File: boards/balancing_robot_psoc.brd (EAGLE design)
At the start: 35 x 75 mm, 31 parts

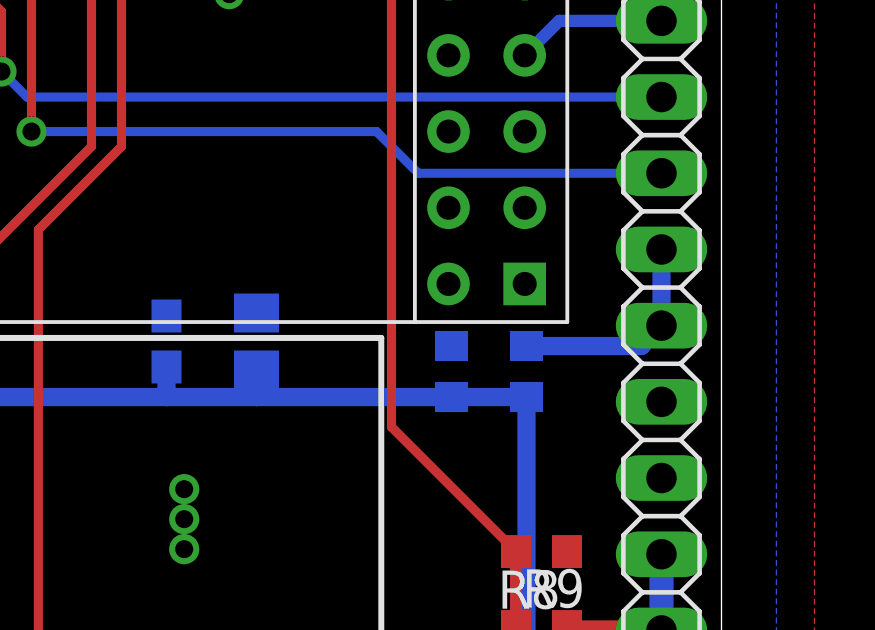
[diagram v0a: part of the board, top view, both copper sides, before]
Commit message: satland production version of boards
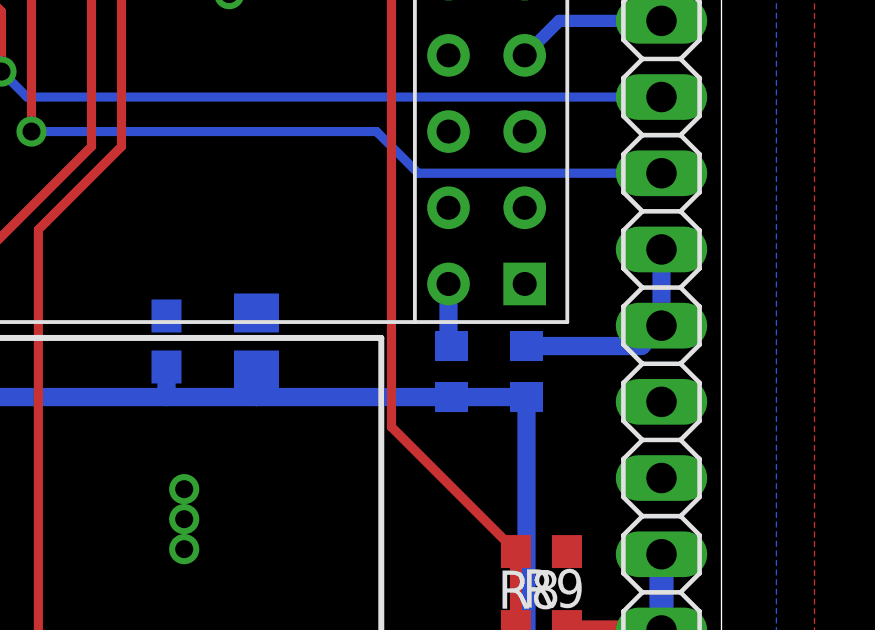
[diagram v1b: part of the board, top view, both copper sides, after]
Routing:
- net N$4: track 0.00 -> 2.17 mm
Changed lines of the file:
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@@
 <param name="mdSmdStop" value="0mil"/>
 <param name="msWidth" value="10mil"/>
-<param name="msDrill" value="24mil"/>
+<param name="msDrill" value="0.05mm"/>
 <param name="msMicroVia" value="9.99mm"/>
 <param name="msBlindViaRatio" value="0.5"/>
@@
 <contactref element="U$1" pad="1.2"/>
 <contactref element="R4" pad="1"/>
-<wire x1="26" y1="22.85" x2="25.9" y2="24.92" width="0" layer="19" extent="16-16"/>
+<wire x1="26" y1="22.85" x2="25.9" y2="22.85" width="0.6096" layer="16"/>
+<wire x1="25.9" y1="22.85" x2="25.9" y2="24.92" width="0.6096" layer="16"/>
 </signal>
 <signal name="POWER_SUP">
